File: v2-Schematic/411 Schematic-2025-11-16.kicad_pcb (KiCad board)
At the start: 2 copper layers, 134.1 x 85.4 mm, 69 parts, among them J1 IMU_Int1_Int2, J2 Screen, J3 Light+, J4 Light-, J5 Light-, J6 Light+, Q1 NMOS, Q2 NMOS, Q3 NMOS, U10 MCP16301x-xCH, U3 TP4056-42-ESOP8, U6 DW01A, U7 MCP1640Bx-xMC, U9 Pico

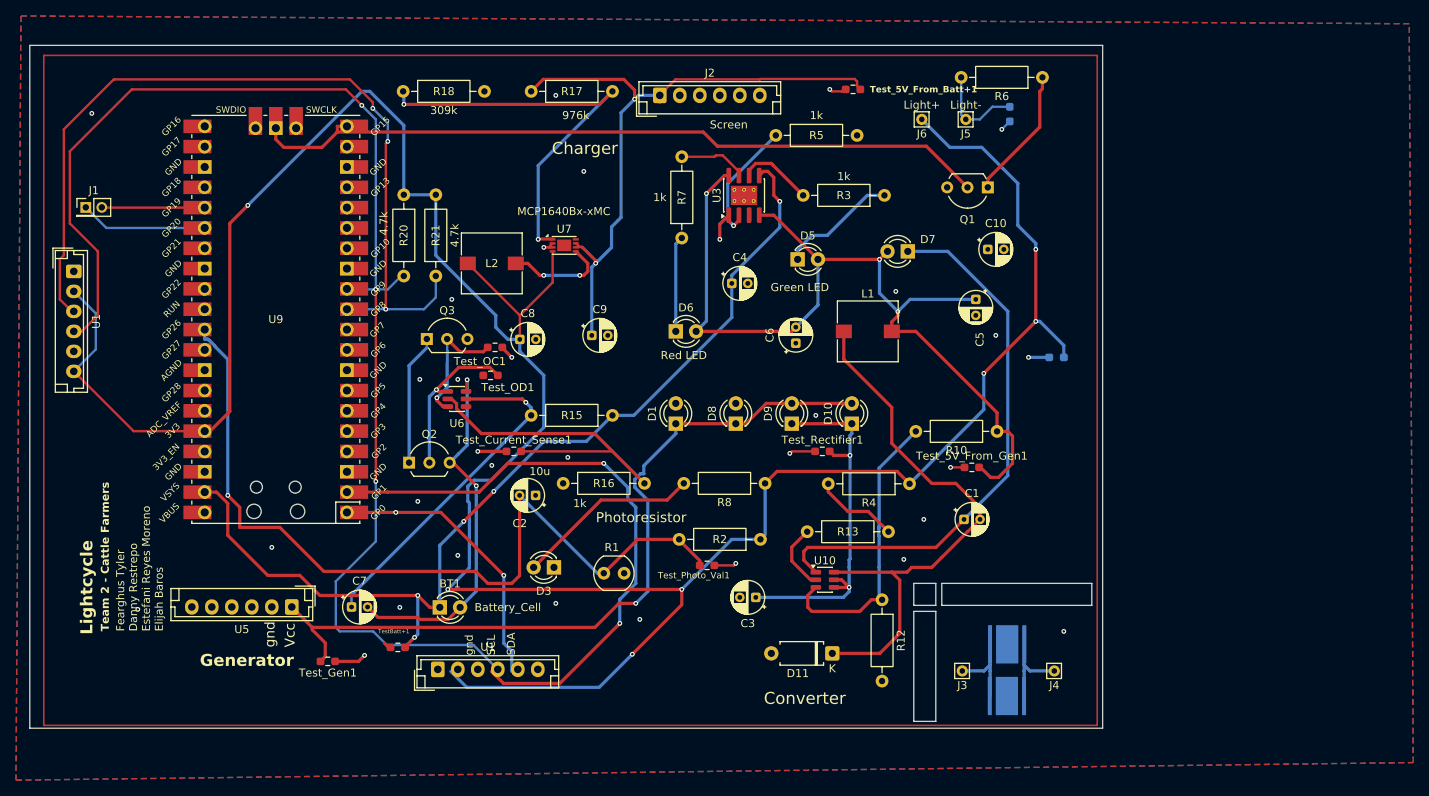
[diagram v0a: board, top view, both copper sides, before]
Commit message: Added v2 and v3 of our project schematic & PCB
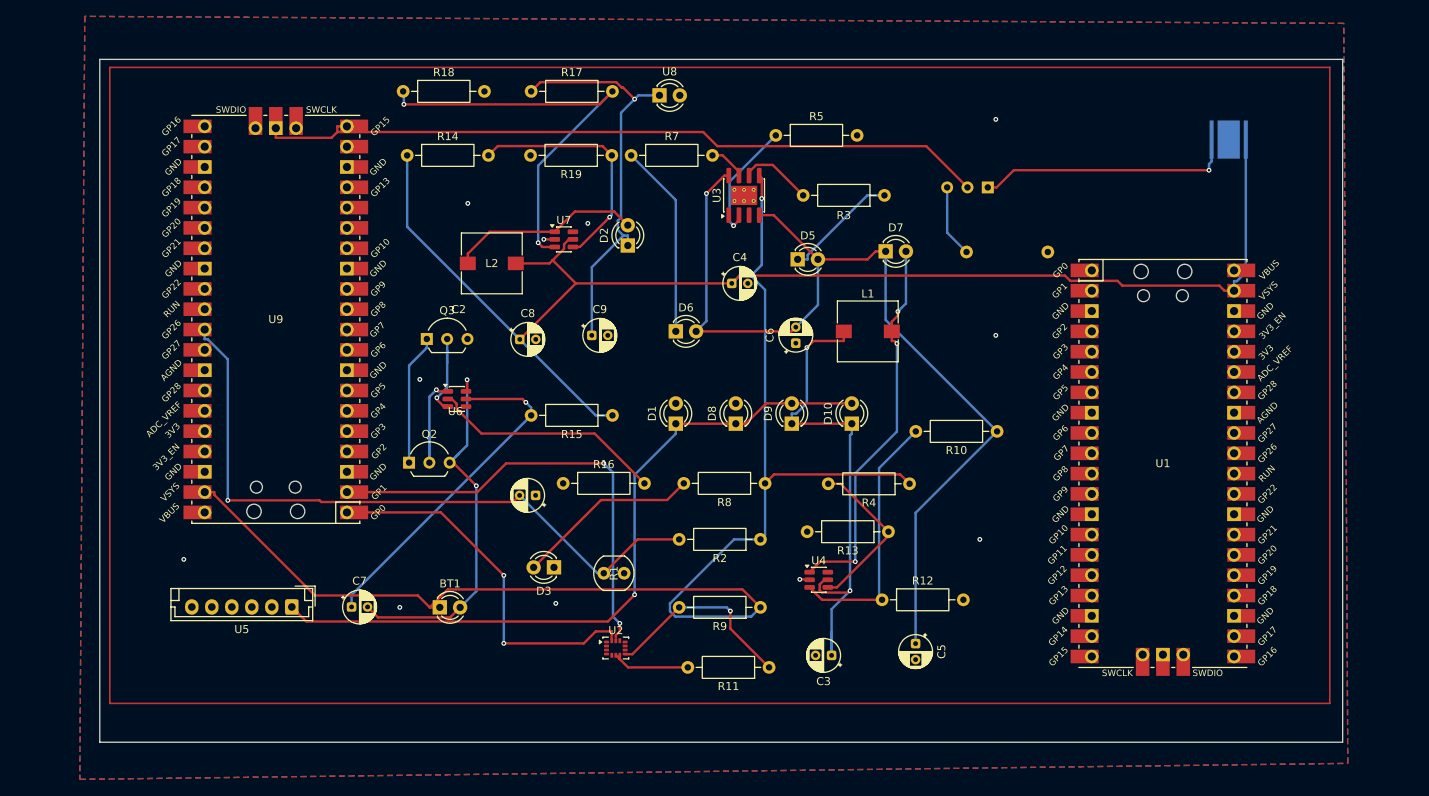
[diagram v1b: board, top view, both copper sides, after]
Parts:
- removed C1, C10: 100n, Capacitor_THT:CP_Radial_D4.0mm_P2.00mm
- removed D11: D_Schottky, Diode_THT:D_A-405_P7.62mm_Horizontal
- removed J1: IMU_Int1_Int2, Connector_PinHeader_2.00mm:PinHeader_2x01_P2.00mm_Vertical
- removed J2: Screen, Connector_JST:JST_EH_B6B-EH-A_1x06_P2.50mm_Vertical
- removed J3, J6: Light+, Connector_Pin:Pin_D0.7mm_L6.5mm_W1.8mm_FlatFork
- removed J4, J5: Light-, Connector_Pin:Pin_D0.7mm_L6.5mm_W1.8mm_FlatFork
- removed R20, R21: 4.7k, Resistor_THT:R_Axial_DIN0207_L6.3mm_D2.5mm_P10.16mm_Horizontal
- removed TestBatt+1, Test_5V_From_Batt+1, Test_5V_From_Gen1, Test_Current_Sense1, Test_Gen1, Test_LED+1, Test_LED-1, Test_OC1, Test_OD1, Test_Photo_Val1, Test_Rectifier1: 0R, Resistor_SMD:R_0603_1608Metric_Pad0.98x0.95mm_HandSolder
- removed the U1 at (102.8, 140.2)
- removed the U1 at (57.2, 90.5)
- removed U10: MCP16301x-xCH, Package_TO_SOT_SMD:SOT-23-6
- added R11: 1k, Resistor_THT:R_Axial_DIN0207_L6.3mm_D2.5mm_P10.16mm_Horizontal, F.Cu at (144.2, 140.0)
- added R14: 1k, Resistor_THT:R_Axial_DIN0207_L6.3mm_D2.5mm_P10.16mm_Horizontal, F.Cu at (98.9, 76.0)
- added R19: 1k, Resistor_THT:R_Axial_DIN0207_L6.3mm_D2.5mm_P10.16mm_Horizontal, F.Cu at (124.5, 76.0)
- added R9: 1k, Resistor_THT:R_Axial_DIN0207_L6.3mm_D2.5mm_P10.16mm_Horizontal, F.Cu at (143.1, 132.5)
- added U1: Pico, MCU_RaspberryPi_and_Boards:RPi_Pico_SMD_TH, F.Cu at (193.4, 114.5)
- added U2: LSM6DS3, Package_LGA:LGA-14_3x2.5mm_P0.5mm_LayoutBorder3x4y, F.Cu at (125.0, 137.6)
- added U4: MT3608, Package_TO_SOT_SMD:SOT-23-6, F.Cu at (150.4, 129.1)
- added U8: ~, LED_THT:LED_D3.0mm_Clear, F.Cu at (130.5, 68.5)
- C5: value 20u -> 100u
- C8: value 4.7u -> 100u
- C9: value 10u -> 100u
- D2: value LED_Cree_XHP50_3V_HighDensity -> 1N4148WT; footprint LED_SMD:LED_Cree-XHP50_3V_HighDensity -> LED_THT:LED_D3.0mm_Clear; moved to F.Cu
- D5: value Green LED -> LED
- D6: value Red LED -> LED
- L1: value 22u -> 1n
- L2: value 4.7u -> 1n
- Q1, R6: moved to B.Cu
- R10: value 52.3k -> 10k
- R17: value 976k -> 3.5k
- R18: value 309k -> 10k
- R5: value 2k -> 1k
- U7: value MCP1640Bx-xMC -> MT3608; footprint Package_DFN_QFN:DFN-8-1EP_3x2mm_P0.5mm_EP1.75x1.45mm -> Package_TO_SOT_SMD:SOT-23-6
- moved D2 73.6 mm to (126.5, 87.3), turned to 90 degrees
- moved D4 68.9 mm to (201.6, 74.0), turned to 0 degrees
- moved C5 43.7 mm to (162.5, 137.0)
- moved R6 21.8 mm to (179.0, 88.1)
- moved R7 12.1 mm to (126.9, 76.0), turned to 0 degrees
- moved C3 11.9 mm to (152.0, 138.5)
- moved D7 2.77 mm to (158.7, 88.0), turned to 0 degrees
- moved U7 0.75 mm to (118.5, 86.5)
- turned L2 to 180 degrees
- turned R12 to 0 degrees
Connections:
- BT1 pad 1: /Batt+ -> 3.7V
- C4 pad 1: /Batt+ -> 3.7V
- C8 pad 1: /Batt+ -> 3.7V
- D2 pad 1: Net-(D2-K) -> /5V
- D4 pad 1: Net-(D2-K) -> Net-(D4-K)
- D4 pad 2: Net-(D2-A) -> 3.7V
- D7 pad 1: Net-(D7-K) -> /V_charge
- D7 pad 2: /V_charge -> Net-(D7-A)
- L1 pad 1: Net-(D11-K) -> Net-(D10-K)
- L1 pad 2: /V_charge -> Net-(D7-A)
- L2 pad 1: /Batt+ -> 3.7V
- L2 pad 2: Net-(U7-SW) -> Net-(D2-A)
- Q1 pad 1: Net-(Q1-D) -> Net-(D4-K)
- Q1 pad 3: GND -> Net-(Q1-S)
- R15 pad 1: /Batt+ -> 3.7V
- R17 pad 2: Net-(U7-V_{FB}) -> Net-(U7-FB)
- R18 pad 1: Net-(U7-V_{FB}) -> Net-(U7-FB)
- R2 pad 1: 3.3V -> 3.7V
- R4 pad 1: 3.3V -> 3.7V
- R6 pad 1: Net-(Q1-D) -> GND
- R6 pad 2: Net-(J5-Pin_1) -> Net-(Q1-S)
- R8 pad 1: 3.3V -> 3.7V
- U3 pad 1: GND -> unconnected-(U3-TEMP-Pad1)
- U3 pad 5: /Batt+ -> 3.7V
- U7 pad 1: Net-(U7-V_{FB}) -> Net-(D2-A)
- U7 pad 3: GND -> Net-(U7-FB)
- U7 pad 4: /Batt+ -> Net-(U7-EN)
- U7 pad 5: Net-(U7-SW) -> 3.7V
- U7 pad 6: /5V -> unconnected-(U7-NC-Pad6)
- U9 pad 1: /GPIO0_TX -> /GPIO0
- U9 pad 11: /GPIO8 -> unconnected-(U9-GPIO8-Pad11)
- U9 pad 12: /GPIO9 -> unconnected-(U9-GPIO9-Pad12)
- U9 pad 2: /GPIO1_RX -> /GPIO1
- U9 pad 25: /GPIO21 -> unconnected-(U9-GPIO19-Pad25)
- U9 pad 26: /GPIO20 -> unconnected-(U9-GPIO20-Pad26)
- U9 pad 32: /GPIO27 -> unconnected-(U9-GPIO27_ADC1-Pad32)_1
- U9 pad 36: 3.3V -> unconnected-(U9-3V3-Pad36)
- U9 pad 39: /Batt+ -> 3.7V
- U9 pad 42: GND -> /GPIO15
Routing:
- net 3.7V: track 0.00 -> 345.7 mm, vias 0 -> 1
- net 3.3V: track 335.3 -> 0.00 mm, vias 7 -> 0
- net /GPIO9: track 164.6 -> 0.00 mm, vias 5 -> 0
- net /Batt+: track 146.0 -> 0.00 mm, vias 5 -> 0
- net (no net): track 111.1 -> 0.00 mm
- net /GPIO8: track 107.4 -> 0.00 mm, vias 3 -> 0
- net Net-(D11-K): track 70.8 -> 0.00 mm
- net Net-(D7-K): track 68.8 -> 0.00 mm
- net /GPIO1: track 0.00 -> 56.4 mm, vias 0 -> 2
- net Net-(U7-FB): track 0.00 -> 53.5 mm, vias 0 -> 2
- net Net-(U7-V_{FB}): track 52.6 -> 0.00 mm, vias 2 -> 0
- net Net-(D7-A): track 0.00 -> 48.4 mm, vias 0 -> 3
- net /GPIO0: track 0.00 -> 46.5 mm, vias 0 -> 2
- net Net-(D4-K): track 0.00 -> 32.5 mm, vias 0 -> 1
- net /5V: track 82.3 -> 51.7 mm, vias 2 -> 1
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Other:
- board size 134.1 x 85.4 mm -> 155.4 x 85.4 mm
- board text removed: "1k"
- board text removed: "Charger"
- board text removed: "Converter"
- board text removed: "Fearghus Tyler Danny Restrepo Estefani Reyes Moreno Elijah Baros"
- board text removed: "Generator"
- board text removed: "Lightcycle"
- board text removed: "Photoresistor"
- board text removed: "SCL"
- board text removed: "SDA"
- board text removed: "Screen"
- board text removed: "Team 2 - Cattle Farmers"
- board text removed: "Vcc"
- board text removed: "gnd"
